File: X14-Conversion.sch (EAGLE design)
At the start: 23 parts, among them P1 282837-2, P2 282837-2, P3 282837-2

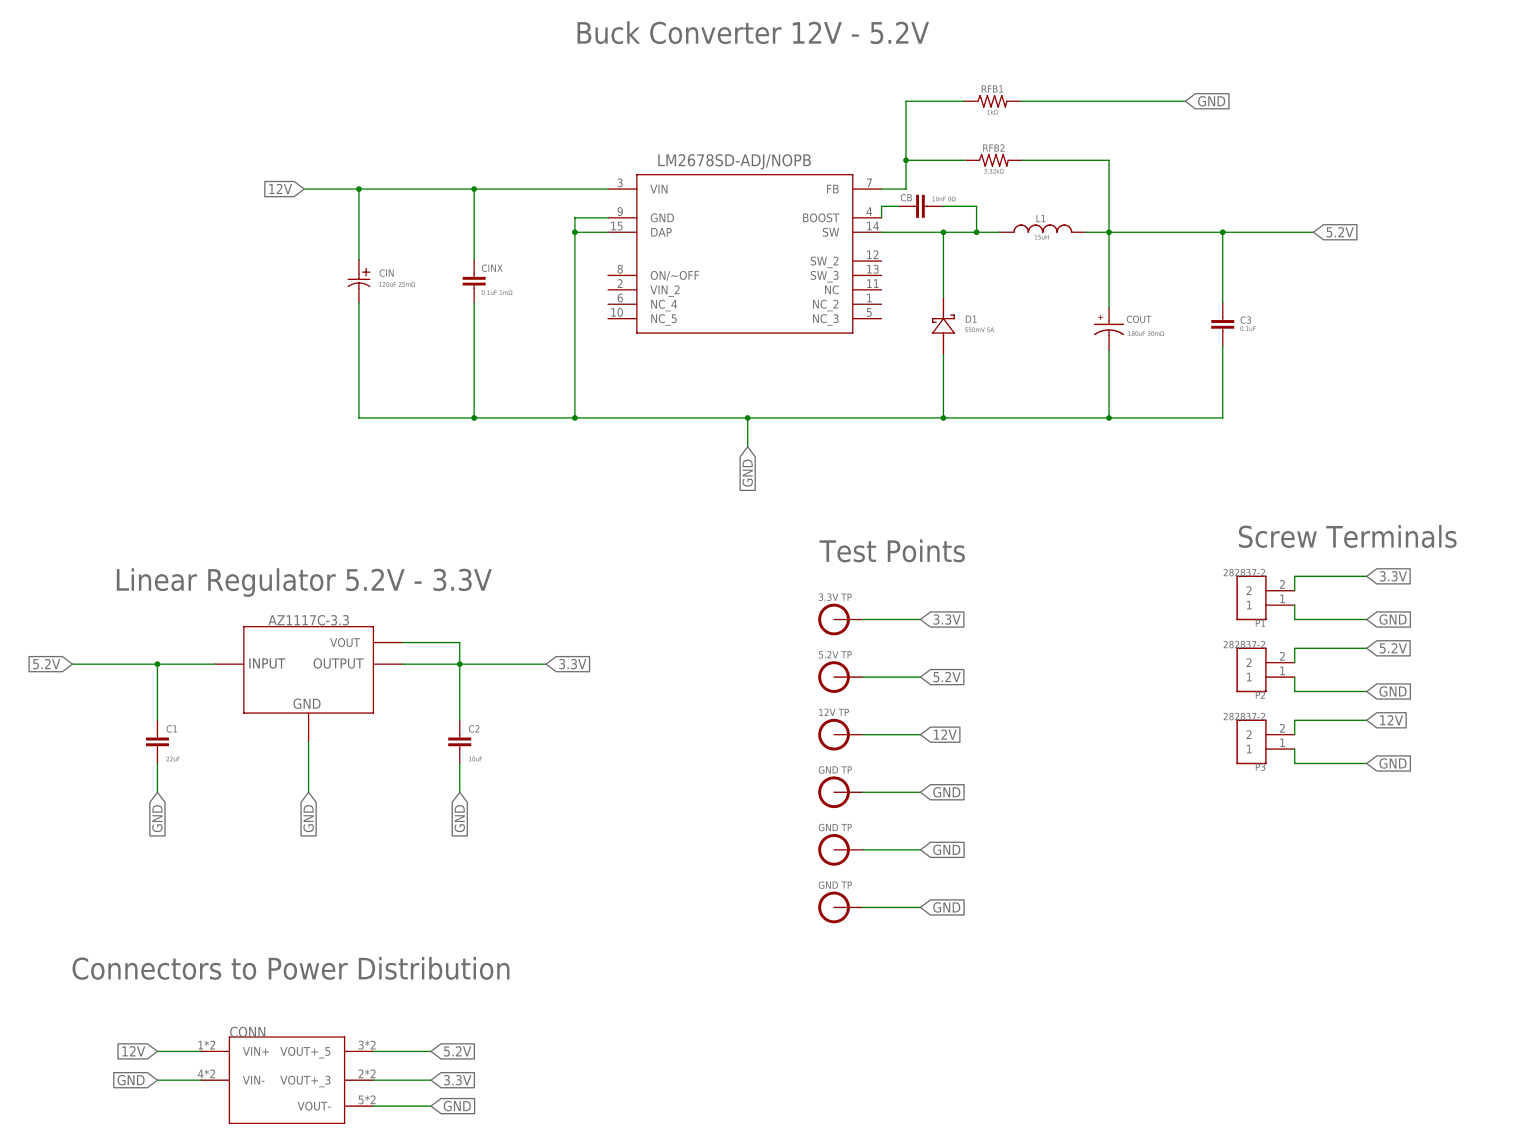
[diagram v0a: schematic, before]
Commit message: Complete Board Layout
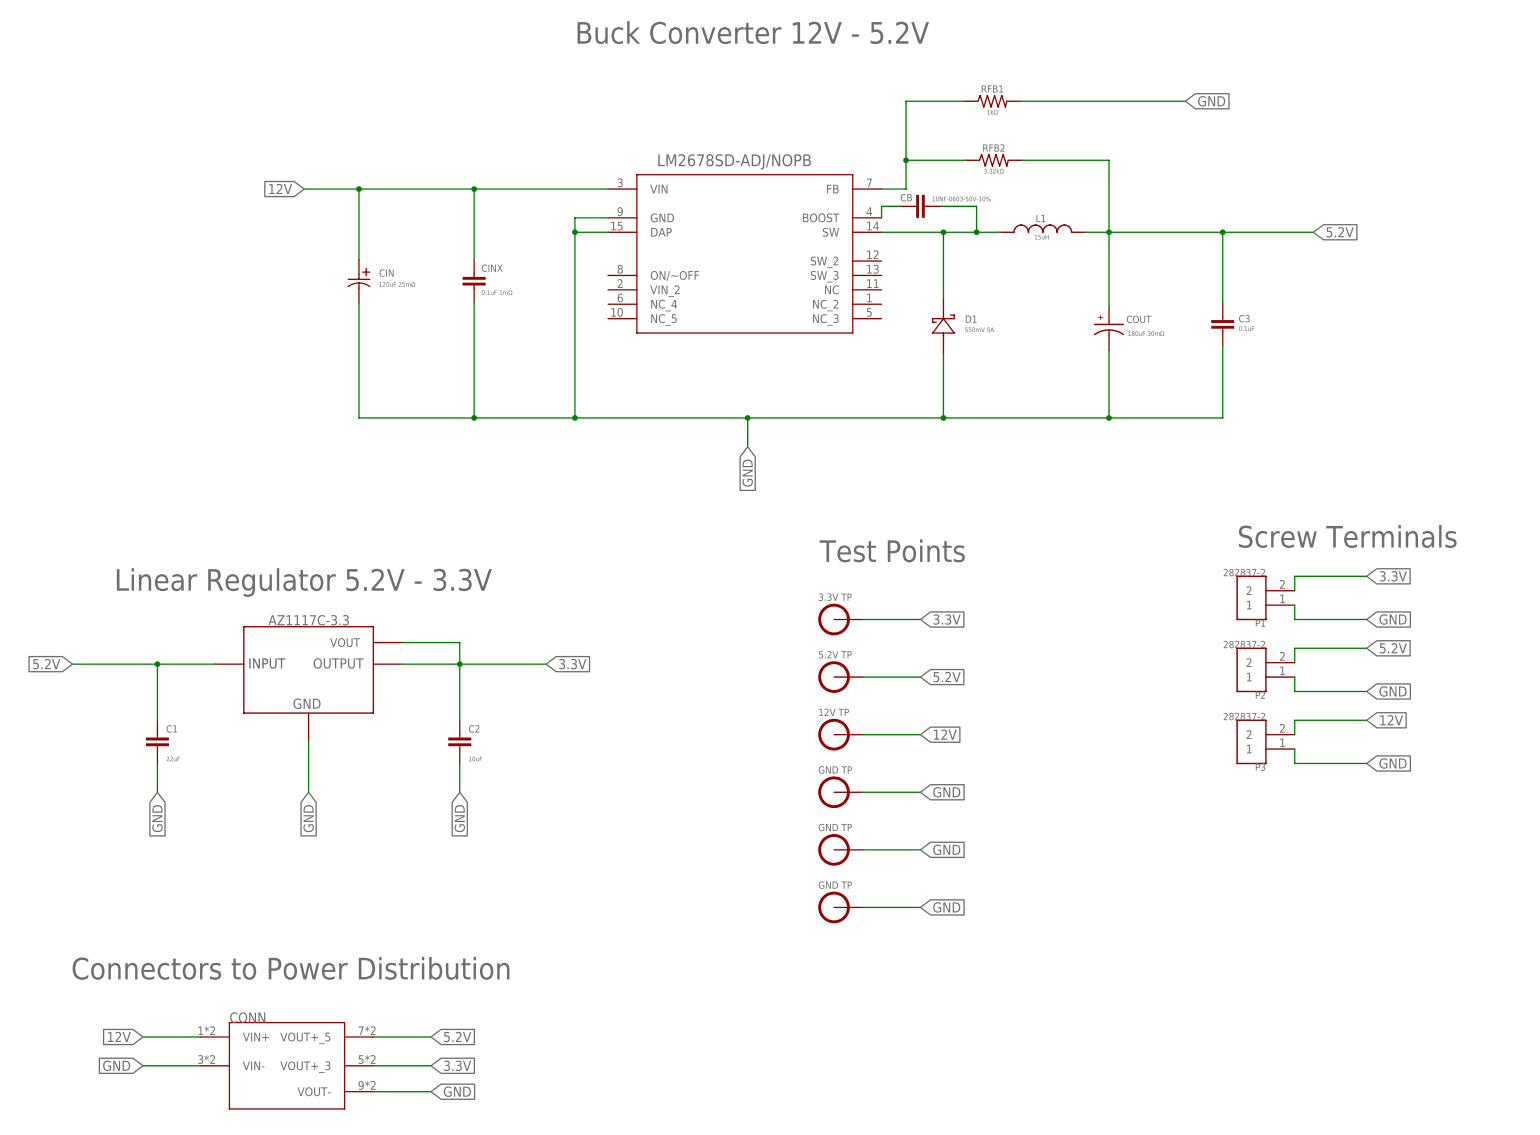
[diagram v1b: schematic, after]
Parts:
- C3: device SparkFun-Capacitors:0.1UF-0402-16V-10% -> SparkFun-Capacitors:0.1UF-0603-25V-(+80/-20%)
- CB: value 10nF 0Ω -> 10NF-0603-50V-10%
- CONN: value DISTRIBUTION-CONVERSION -> CONVERSION-DISTRIBUTION; device CONN, Distribution-Conversion:DISTRIBUTION-CONVERSION -> CONN, Distribution-Conversion (3):CONVERSION-DISTRIBUTION
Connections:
- net 12V: now also P3.2; no longer P2.2
- net 5.2V: now also P2.2; no longer P1.1
- net GND: now also P1.1; no longer P3.2
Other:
- moved on the sheet: CONN
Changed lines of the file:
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@@
 <part name="FRAME1" library="frames" library_urn="urn:adsk.eagle:library:229" deviceset="A3L-LOC" device=""/>
 <part name="AZ1117C" library="AZ1117C-3.3" deviceset="SOT150P410X160-3N" device="" value="AZ1117C-3.3"/>
-<part name="CONN" library="CONN, Distribution-Conversion" deviceset="DISTRIBUTION-CONVERSION" device=""/>
 <part name="LM2678" library="LM2678SX-ADJNOPB" deviceset="LM2678SD-ADJ/NOPB" device=""/>
 <part name="U$2" library="testpoints" deviceset="3.3V_TESTPOINT" device=""/>
@@
 <part name="P2" library="ScrewPoints_282837-2" deviceset="282837-2" device=""/>
 <part name="P3" library="ScrewPoints_282837-2" deviceset="282837-2" device=""/>
-<part name="C3" library="SparkFun-Capacitors" library_urn="urn:adsk.eagle:library:510" deviceset="0.1UF" device="-0402-16V-10%" package3d_urn="urn:adsk.eagle:package:37413/1" value="0.1uF"/>
 <part name="RFB2" library="SparkFun-Resistors" library_urn="urn:adsk.eagle:library:532" deviceset="3.3KOHM" device="-0603-1/10W-1%" package3d_urn="urn:adsk.eagle:package:39650/1" value="3.32kΩ"/>
 <part name="RFB1" library="SparkFun-Resistors" library_urn="urn:adsk.eagle:library:532" deviceset="1KOHM" device="-0603-1/10W-1%" package3d_urn="urn:adsk.eagle:package:39650/1" value="1kΩ"/>
-<part name="CB" library="SparkFun-Capacitors" library_urn="urn:adsk.eagle:library:510" deviceset="10NF" device="-0603-50V-10%" package3d_urn="urn:adsk.eagle:package:37414/1" value="10nF 0Ω"/>
+<part name="CB" library="SparkFun-Capacitors" library_urn="urn:adsk.eagle:library:510" deviceset="10NF" device="-0603-50V-10%" package3d_urn="urn:adsk.eagle:package:37414/1" value="10NF-0603-50V-10%"/>
 <part name="CINX" library="SparkFun-Capacitors" library_urn="urn:adsk.eagle:library:510" deviceset="0.1UF" device="-0603-25V-(+80/-20%)" package3d_urn="urn:adsk.eagle:package:37414/1" value="0.1uF 1mΩ"/>
 <part name="C2" library="SparkFun-Capacitors" library_urn="urn:adsk.eagle:library:510" deviceset="10UF" device="-0603-6.3V-20%" package3d_urn="urn:adsk.eagle:package:37414/1" value="10uF"/>
@@
 <part name="D1" library="CDBC520-G_Library" deviceset="CDBG520-G" device="" value="550mV 5A"/>
 <part name="CIN" library="20SVPF120M" deviceset="20SVPF120M" device="" value="120uF 25mΩ"/>
+<part name="C3" library="SparkFun-Capacitors" library_urn="urn:adsk.eagle:library:510" deviceset="0.1UF" device="-0603-25V-(+80/-20%)" package3d_urn="urn:adsk.eagle:package:37414/1" value="0.1uF"/>
+<part name="CONN" library="CONN, Distribution-Conversion (3)" deviceset="CONVERSION-DISTRIBUTION" device=""/>
 </parts>
 <sheets>
@@
 </instance>
 <instance part="AZ1117C" gate="G$1" x="-75.692" y="-10.668" smashed="yes"/>
-<instance part="CONN" gate="G$1" x="-81.28" y="-83.82" smashed="yes">
-<attribute name="NAME" x="-88.9" y="-76.2" size="1.778" layer="95"/>
-</instance>
 <instance part="LM2678" gate="A" x="-2.54" y="66.04" smashed="yes">
 <attribute name="NAME" x="-13.6144" y="79.9846" size="2.0828" layer="95" ratio="6" rot="SR0" display="off"/>
@@
 <attribute name="VALUE" x="93.98236875" y="-19.025490625" size="1.274909375" layer="96" rot="R180"/>
 </instance>
-<instance part="C3" gate="G$1" x="86.36" y="48.26" smashed="yes">
-<attribute name="NAME" x="89.408" y="49.657" size="1.27" layer="95"/>
-<attribute name="VALUE" x="89.408" y="48.387" size="0.8128" layer="96"/>
-</instance>
 <instance part="RFB2" gate="G$1" x="45.974" y="78.486" smashed="yes">
 <attribute name="NAME" x="45.974" y="80.01" size="1.27" layer="95" align="bottom-center"/>
@@
 <attribute name="VALUE" x="-62.5571" y="56.1721" size="0.8128" layer="96" ratio="10"/>
 <attribute name="NAME" x="-62.5048" y="57.9501" size="1.27" layer="95" ratio="10"/>
+</instance>
+<instance part="C3" gate="G$1" x="86.36" y="48.26" smashed="yes">
+<attribute name="NAME" x="89.154" y="49.911" size="1.27" layer="95"/>
+<attribute name="VALUE" x="89.154" y="48.387" size="0.8128" layer="96"/>
+</instance>
+<instance part="CONN" gate="G$1" x="-81.28" y="-81.28" smashed="yes">
+<attribute name="NAME" x="-88.9" y="-73.66" size="1.778" layer="95"/>
 </instance>
 </instances>
@@
 <label x="-48.26" y="-33.02" size="1.778" layer="95" rot="R270" xref="yes"/>
 <pinref part="C2" gate="G$1" pin="2"/>
-</segment>
-<segment>
-<pinref part="CONN" gate="G$1" pin="VOUT-"/>
-<wire x1="-63.5" y1="-88.392" x2="-53.34" y2="-88.392" width="0.1524" layer="91"/>
-<label x="-53.34" y="-88.392" size="1.778" layer="95" xref="yes"/>
-</segment>
-<segment>
-<pinref part="CONN" gate="G$1" pin="VIN-"/>
-<wire x1="-93.98" y1="-83.82" x2="-101.6" y2="-83.82" width="0.1524" layer="91"/>
-<label x="-101.6" y="-83.82" size="1.778" layer="95" rot="R180" xref="yes"/>
 </segment>
 <segment>
@@
 <wire x1="-66.04" y1="33.02" x2="-66.04" y2="53.34" width="0.1524" layer="91"/>
 <junction x="-45.72" y="33.02"/>
-<pinref part="C3" gate="G$1" pin="2"/>
 <wire x1="66.294" y1="33.02" x2="86.36" y2="33.02" width="0.1524" layer="91"/>
 <wire x1="86.36" y1="33.02" x2="86.36" y2="45.72" width="0.1524" layer="91"/>
@@
 <pinref part="D1" gate="A" pin="2"/>
 <pinref part="CIN" gate="G$1" pin="2"/>
+<pinref part="C3" gate="G$1" pin="2"/>
 </segment>
 <segment>
@@
 </segment>
 <segment>
-<pinref part="P3" gate="G$1" pin="2"/>
-<wire x1="99.06" y1="-22.86" x2="99.06" y2="-20.32" width="0.1524" layer="91"/>
-</segment>
-<segment>
 <pinref part="P3" gate="G$1" pin="1"/>
 <wire x1="99.06" y1="-25.4" x2="99.06" y2="-27.94" width="0.1524" layer="91"/>
@@
 <wire x1="99.06" y1="-2.54" x2="111.76" y2="-2.54" width="0.1524" layer="91"/>
 <label x="111.76" y="-2.54" size="1.778" layer="95" xref="yes"/>
+<pinref part="P1" gate="G$1" pin="1"/>
+<wire x1="99.06" y1="-2.54" x2="99.06" y2="0" width="0.1524" layer="91"/>
+</segment>
+<segment>
+<pinref part="CONN" gate="G$1" pin="VIN-"/>
+<wire x1="-93.98" y1="-81.28" x2="-104.14" y2="-81.28" width="0.1524" layer="91"/>
+<label x="-104.14" y="-81.28" size="1.778" layer="95" rot="R180" xref="yes"/>
+</segment>
+<segment>
+<pinref part="CONN" gate="G$1" pin="VOUT-"/>
+<wire x1="-63.5" y1="-85.852" x2="-53.34" y2="-85.852" width="0.1524" layer="91"/>
+<label x="-53.34" y="-85.852" size="1.778" layer="95" xref="yes"/>
 </segment>
 </net>
@@
 </segment>
 <segment>
-<pinref part="CONN" gate="G$1" pin="VOUT+_3"/>
-<wire x1="-63.5" y1="-83.82" x2="-53.34" y2="-83.82" width="0.1524" layer="91"/>
-<label x="-53.34" y="-83.82" size="1.778" layer="95" xref="yes"/>
-</segment>
-<segment>
 <pinref part="U$2" gate="G$1" pin="3.3V"/>
 <wire x1="22.86" y1="-2.54" x2="33.02" y2="-2.54" width="0.1524" layer="91"/>
@@
 <wire x1="99.06" y1="5.08" x2="111.76" y2="5.08" width="0.1524" layer="91"/>
 <label x="111.76" y="5.08" size="1.778" layer="95" xref="yes"/>
+</segment>
+<segment>
+<pinref part="CONN" gate="G$1" pin="VOUT+_3"/>
+<wire x1="-63.5" y1="-81.28" x2="-53.34" y2="-81.28" width="0.1524" layer="91"/>
+<label x="-53.34" y="-81.28" size="1.778" layer="95" xref="yes"/>
 </segment>
 </net>
@@
 <label x="-116.586" y="-10.414" size="1.778" layer="95" rot="R180" xref="yes"/>
 <pinref part="C1" gate="G$1" pin="1"/>
-</segment>
-<segment>
-<pinref part="CONN" gate="G$1" pin="VOUT+_5"/>
-<wire x1="-63.5" y1="-78.74" x2="-53.34" y2="-78.74" width="0.1524" layer="91"/>
-<label x="-53.34" y="-78.74" size="1.778" layer="95" xref="yes"/>
 </segment>
 <segment>
@@
 <label x="102.362" y="65.786" size="1.778" layer="95" xref="yes"/>
 <wire x1="102.362" y1="65.786" x2="86.36" y2="65.786" width="0.1524" layer="91"/>
-<pinref part="C3" gate="G$1" pin="1"/>
 <wire x1="86.36" y1="65.786" x2="66.294" y2="65.786" width="0.1524" layer="91"/>
 <wire x1="86.36" y1="53.34" x2="86.36" y2="65.786" width="0.1524" layer="91"/>
 <junction x="86.36" y="65.786"/>
 <pinref part="RFB2" gate="G$1" pin="2"/>
+<pinref part="C3" gate="G$1" pin="1"/>
 </segment>
 <segment>
@@
 </segment>
 <segment>
-<pinref part="P1" gate="G$1" pin="1"/>
-<wire x1="99.06" y1="0" x2="99.06" y2="-2.54" width="0.1524" layer="91"/>
-</segment>
-<segment>
 <wire x1="99.06" y1="-7.62" x2="111.76" y2="-7.62" width="0.1524" layer="91"/>
 <label x="111.76" y="-7.62" size="1.778" layer="95" xref="yes"/>
+<pinref part="P2" gate="G$1" pin="2"/>
+<wire x1="99.06" y1="-10.16" x2="99.06" y2="-7.62" width="0.1524" layer="91"/>
+</segment>
+<segment>
+<pinref part="CONN" gate="G$1" pin="VOUT+_5"/>
+<wire x1="-63.5" y1="-76.2" x2="-53.34" y2="-76.2" width="0.1524" layer="91"/>
+<label x="-53.34" y="-76.2" size="1.778" layer="95" xref="yes"/>
 </segment>
 </net>
 <net name="12V" class="0">
-<segment>
-<pinref part="CONN" gate="G$1" pin="VIN+"/>
-<wire x1="-93.98" y1="-78.74" x2="-101.6" y2="-78.74" width="0.1524" layer="91"/>
-<label x="-101.6" y="-78.74" size="1.778" layer="95" rot="R180" xref="yes"/>
-</segment>
 <segment>
 <pinref part="LM2678" gate="A" pin="VIN"/>
@@
 </segment>
 <segment>
-<pinref part="P2" gate="G$1" pin="2"/>
-<wire x1="99.06" y1="-10.16" x2="99.06" y2="-7.62" width="0.1524" layer="91"/>
-</segment>
-<segment>
 <wire x1="99.06" y1="-20.32" x2="111.76" y2="-20.32" width="0.1524" layer="91"/>
 <label x="111.76" y="-20.32" size="1.778" layer="95" xref="yes"/>
+<pinref part="P3" gate="G$1" pin="2"/>
+<wire x1="99.06" y1="-20.32" x2="99.06" y2="-22.86" width="0.1524" layer="91"/>
+</segment>
+<segment>
+<pinref part="CONN" gate="G$1" pin="VIN+"/>
+<wire x1="-93.98" y1="-76.2" x2="-104.14" y2="-76.2" width="0.1524" layer="91"/>
+<label x="-104.14" y="-76.2" size="1.778" layer="95" rot="R180" xref="yes"/>
 </segment>
 </net>
